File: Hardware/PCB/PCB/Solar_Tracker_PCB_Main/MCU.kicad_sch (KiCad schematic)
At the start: 13 parts, among them IC1 ESP32-S3-WROOM-1-N4R8, IC5 LM1117MPX-3.3_NOPB, J2 USB4940-00-A

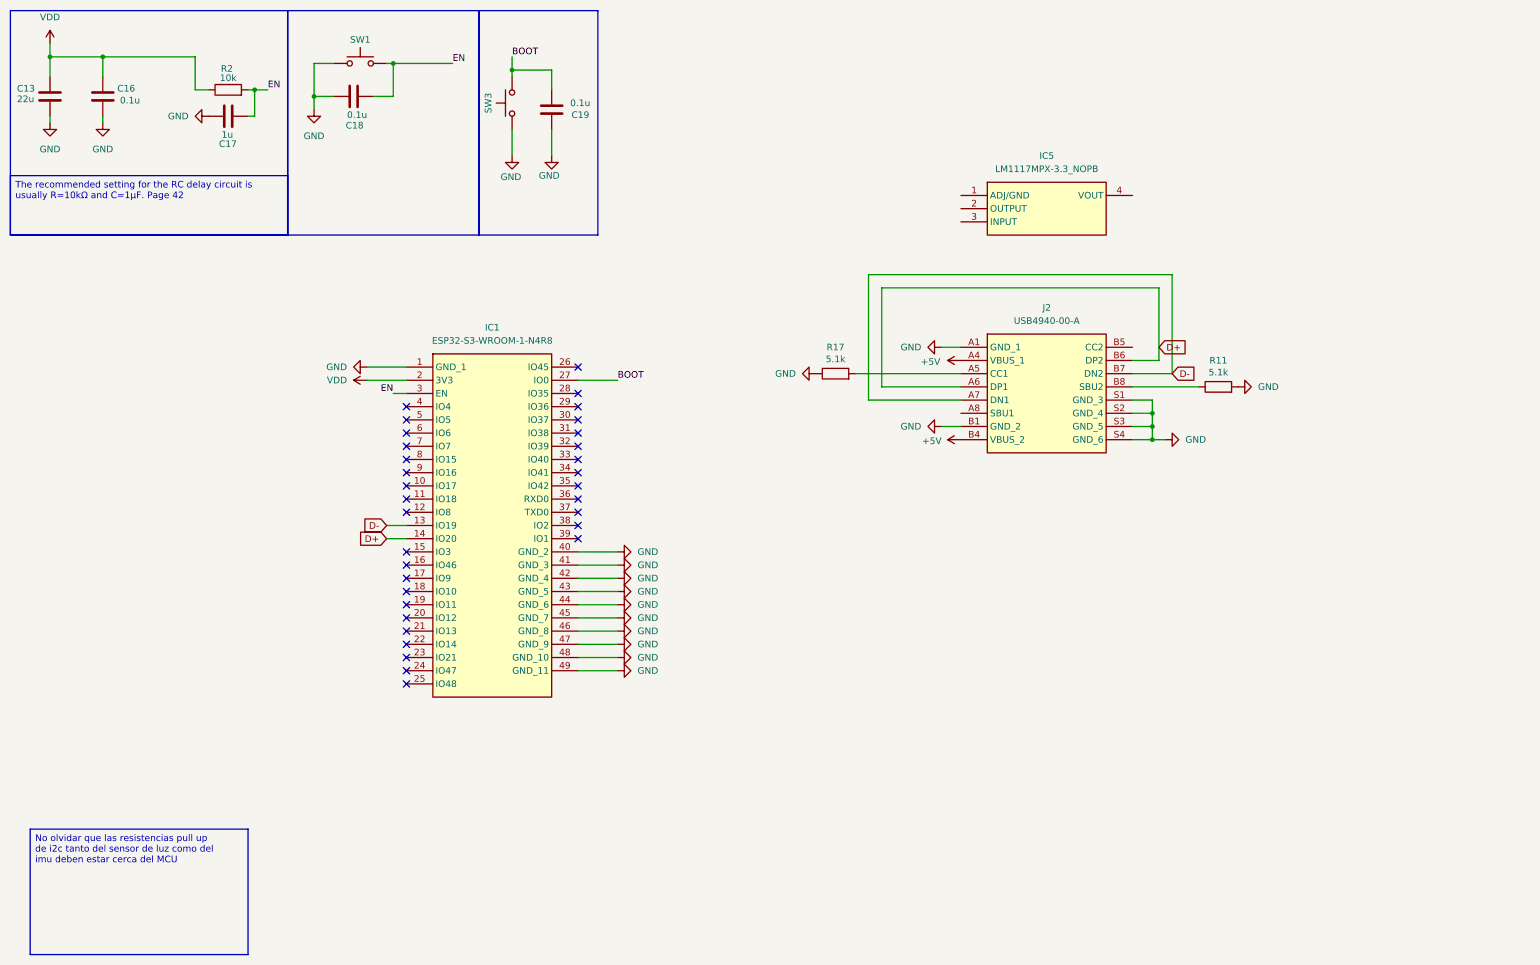
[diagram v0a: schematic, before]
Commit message: Actualizacion Main pcb
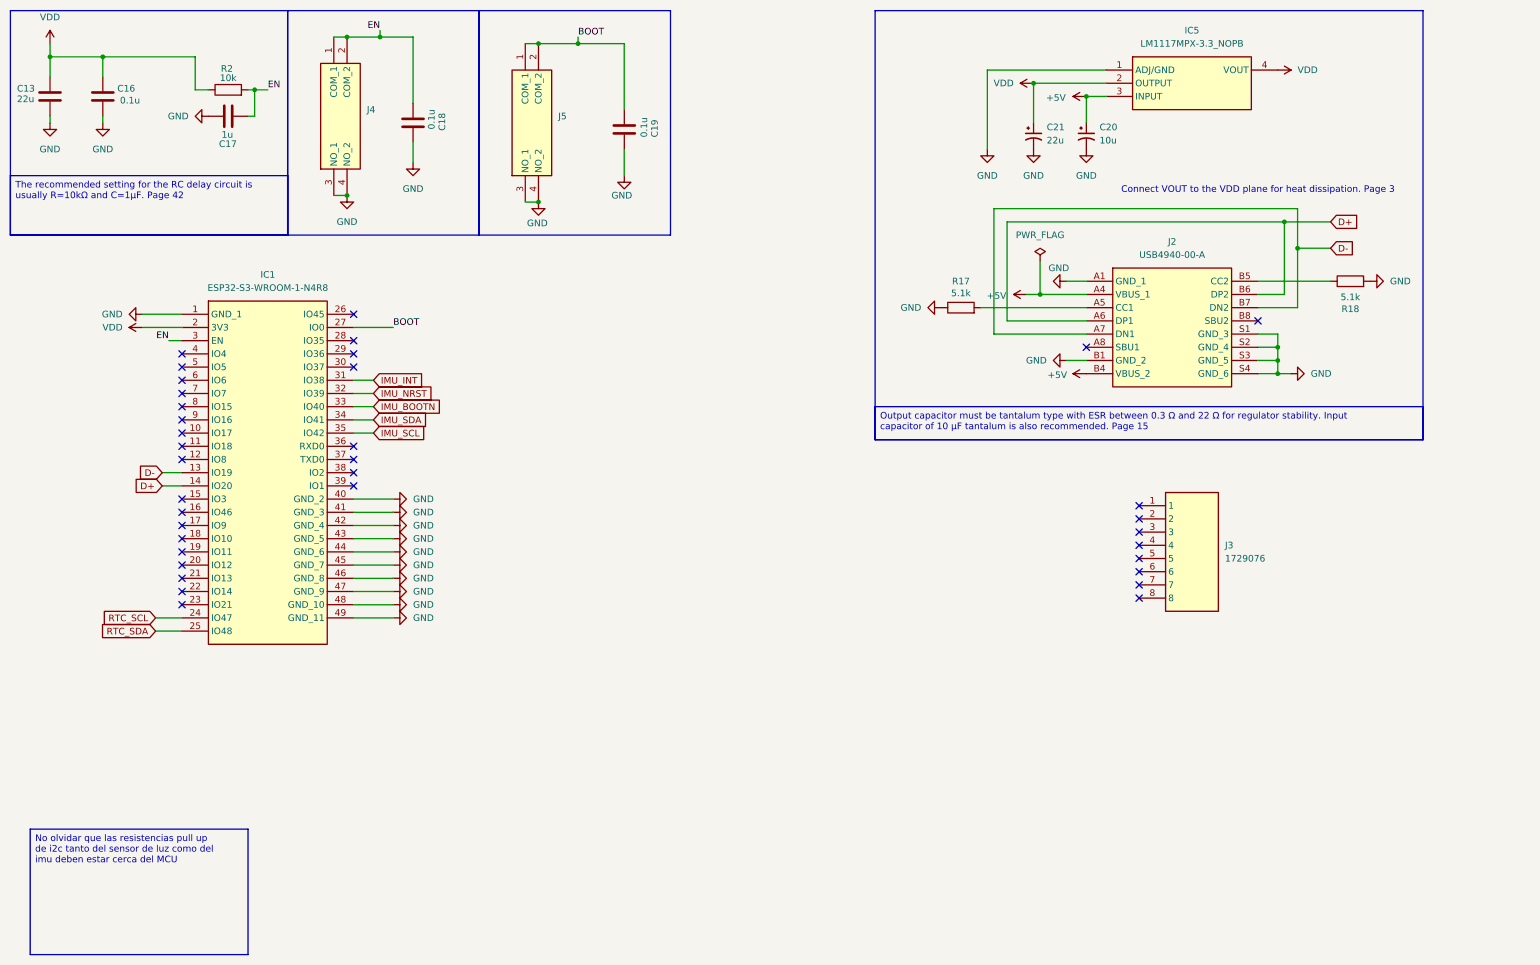
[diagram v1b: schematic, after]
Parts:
- removed R11: 5.1k, symbol Device:R
- removed SW1, SW3: ~, symbol Switch:SW_MEC_5G
- added C20: 10u, Capacitor_SMD:C_0805_2012Metric_Pad1.18x1.45mm_HandSolder, symbol Device:C_Polarized_Small_US
- added C21: 22u, Capacitor_SMD:C_0805_2012Metric_Pad1.18x1.45mm_HandSolder, symbol Device:C_Polarized_Small_US
- added J3: 1729076, 1729076:1729076, symbol 1729076:1729076
- added J4, J5: 1977223-1, 1977223:19772231, symbol 1977223-1:1977223-1
- added R18: 5.1k, Resistor_SMD:R_0805_2012Metric_Pad1.20x1.40mm_HandSolder, symbol Device:R
- R17: footprint (none) -> Resistor_SMD:R_0805_2012Metric_Pad1.20x1.40mm_HandSolder
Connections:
- net +5V: now also IC5.3 (INPUT), C20.1
- net BOOT: now also J5.1 (COM_1), J5.2 (COM_2)
- net EN: now also J4.1 (COM_1), J4.2 (COM_2)
- net GND: now also IC5.1 (ADJ/GND), C20.2, C21.2, J4.3 (NO_1), J4.4 (NO_2), J5.3 (NO_1), J5.4 (NO_2), R18.2
- net VDD: now also IC5.2 (OUTPUT), IC5.4 (VOUT), C21.1
- net RTC_SCL: now reaches IC1.24 (IO47)
- net RTC_SDA: now reaches IC1.25 (IO48)
- net IMU_INT: now reaches IC1.31 (IO38)
- net IMU_NRST: now reaches IC1.32 (IO39)
- net IMU_BOOTN: now reaches IC1.33 (IO40)
- net IMU_SDA: now reaches IC1.34 (IO41)
- net IMU_SCL: now reaches IC1.35 (IO42)
- net at J2.B5 (CC2): now also R18.1
- no-connect marks 33 -> 36
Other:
- note added: "Connect VOUT to the VDD plane for heat dissipation. Page 3"
- moved on the sheet: C18, C19, IC1, IC5, J2, R17
